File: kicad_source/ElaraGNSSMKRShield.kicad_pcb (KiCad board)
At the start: 2 copper layers, 60 x 24 mm, 36 parts, among them CN1 ARDUINO_MKR, CN2 60312202114509, Q1 BSS138, Q2 BSS138, U1 TPS736XX, U2 WIRL-POSI_Elara-I, U3 PCA9306, U4 SN74LVC2G34

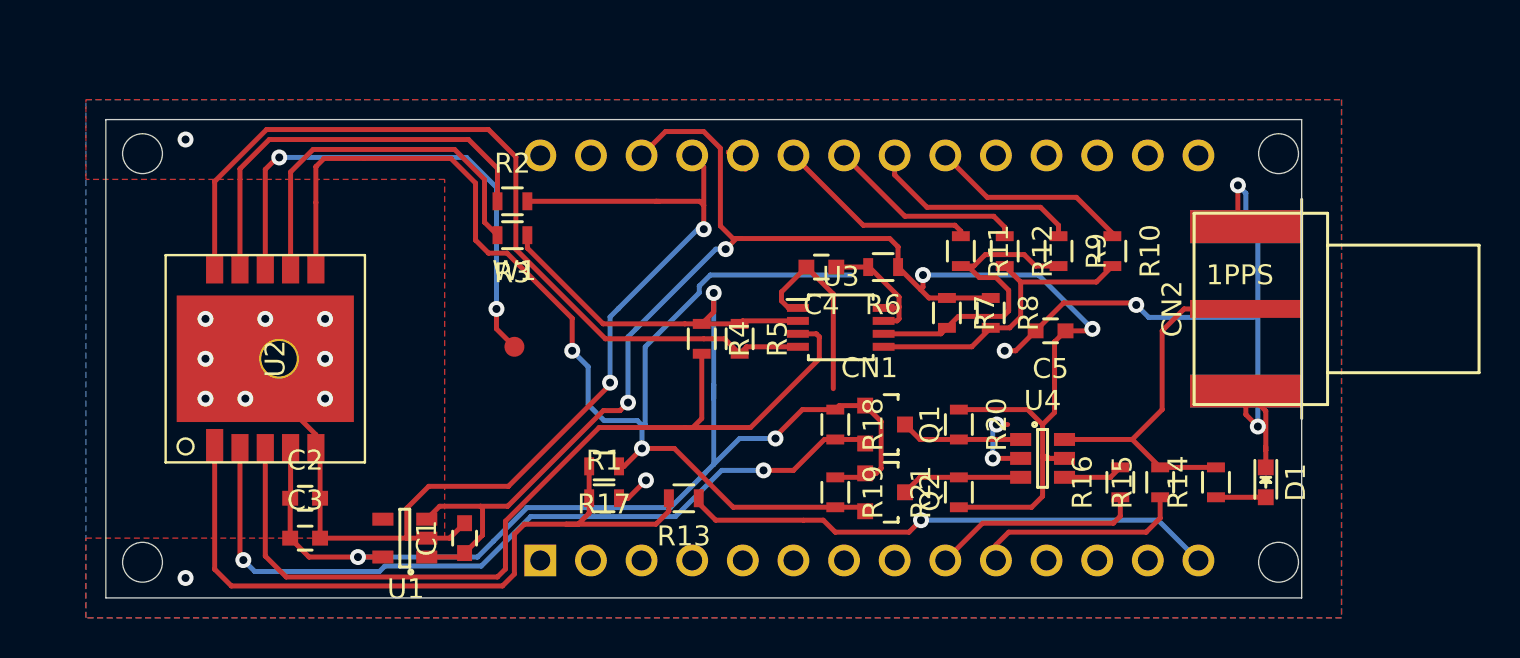
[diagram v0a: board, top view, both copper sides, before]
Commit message: beautified layout, added images, updated files
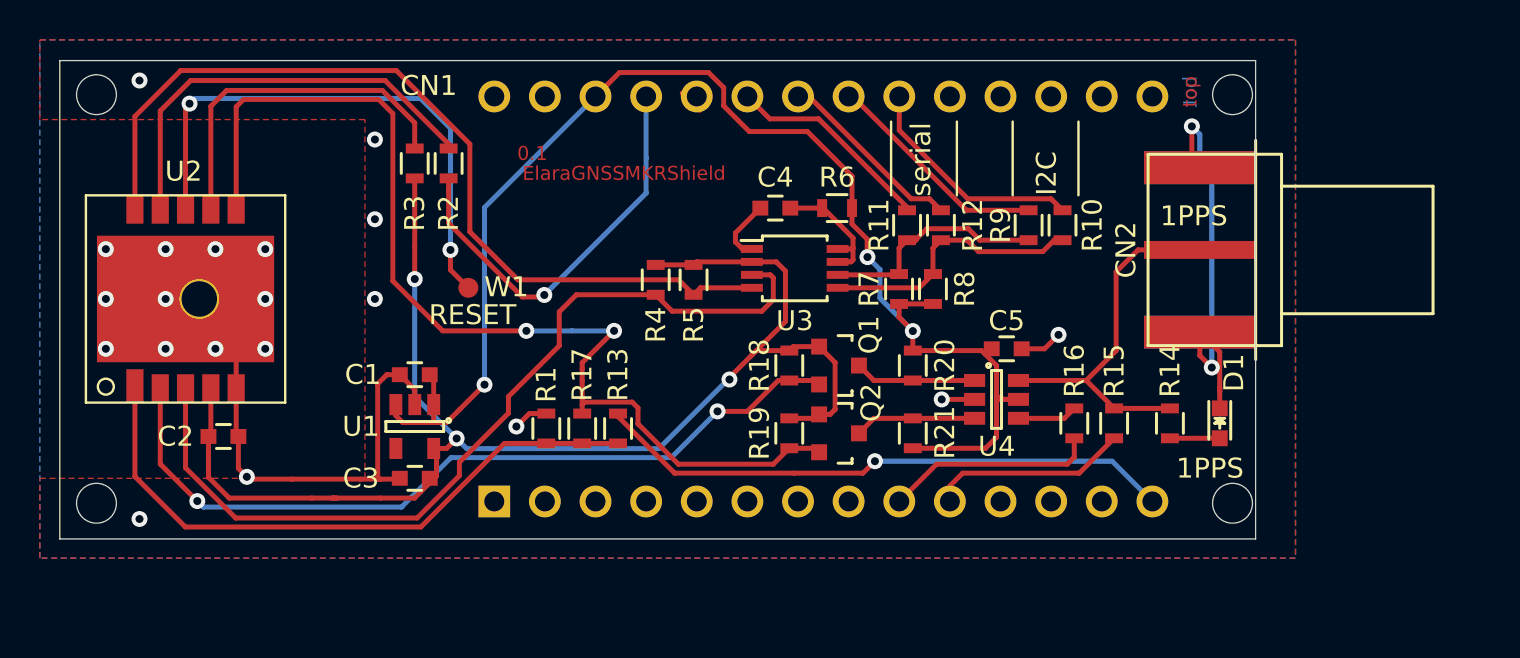
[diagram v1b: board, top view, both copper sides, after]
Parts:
- added L1: Label, labels:generationmake_small_solder, F.Cu at (139.5, 128.6)
- CN1: footprint MODULE_compute:ARDUINO_MKR_HOLES -> MODULE_compute:ARDUINO_MKR_HOLES_PINHEADER
- moved C1 8.57 mm to (129.5, 133.8), turned to 180 degrees
- moved C3 6.26 mm to (129.5, 139.0), turned to 180 degrees
- moved R3 6.08 mm to (129.5, 123.2), turned to 90 degrees
- moved U1 5.62 mm to (129.5, 136.4), turned to 270 degrees
- moved C2 5.14 mm to (119.9, 136.9)
- moved U2 5.00 mm to (118.0, 130.0)
- moved R13 4.81 mm to (139.7, 136.5), turned to 270 degrees
- moved R1 4.55 mm to (136.1, 136.5), turned to 90 degrees
- moved C4 3.75 mm to (147.6, 125.4)
- moved CN1 3.75 mm to (150.0, 130.0)
- moved Q1 3.75 mm to (150.8, 133.3)
- moved R18 3.75 mm to (148.3, 133.3)
- moved R20 3.75 mm to (154.5, 133.3)
- moved R4 3.75 mm to (141.6, 129.0)
- moved R5 3.75 mm to (143.5, 129.0)
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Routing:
- net GND: track 105.6 -> 77.0 mm, vias 19 -> 23
- net +3V3: track 84.8 -> 69.7 mm, vias 4 -> 3
- net /WAKE_UP_1V8: track 62.4 -> 52.9 mm
- net /ON_OFF_1V8: track 36.4 -> 31.6 mm
- net /I2C_CLK_TX: track 16.1 -> 11.3 mm
- net /ON_OFF: track 27.0 -> 29.2 mm
- net /I2C_CLK_1V8: track 45.7 -> 43.9 mm
- net /I2C_DAT_RX: track 15.3 -> 13.5 mm
- net /RESET: track 25.9 -> 27.6 mm
- net /I2C_DAT_1V8: track 42.3 -> 44.0 mm
- net /I2C_DAT: track 10.1 -> 11.6 mm
- net /CTS: track 18.8 -> 17.7 mm
- net /RTS: track 20.8 -> 21.6 mm
- net /1PPS: track 10.6 -> 10.0 mm
- net /I2C_CLK: track 10.8 -> 11.4 mm
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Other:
- board text added: "0.1"
- board text added: "ElaraGNSSMKRShield"
- board text added: "I2C"
- board text added: "RESET"
- board text added: "bot"
- board text added: "serial"
- board text added: "top"
